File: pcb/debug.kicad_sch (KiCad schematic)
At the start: 23 parts, among them J2 USB_B_Micro, SW1 SW_DIP_x02, U2 FT4222HQ, Y1 12MHz

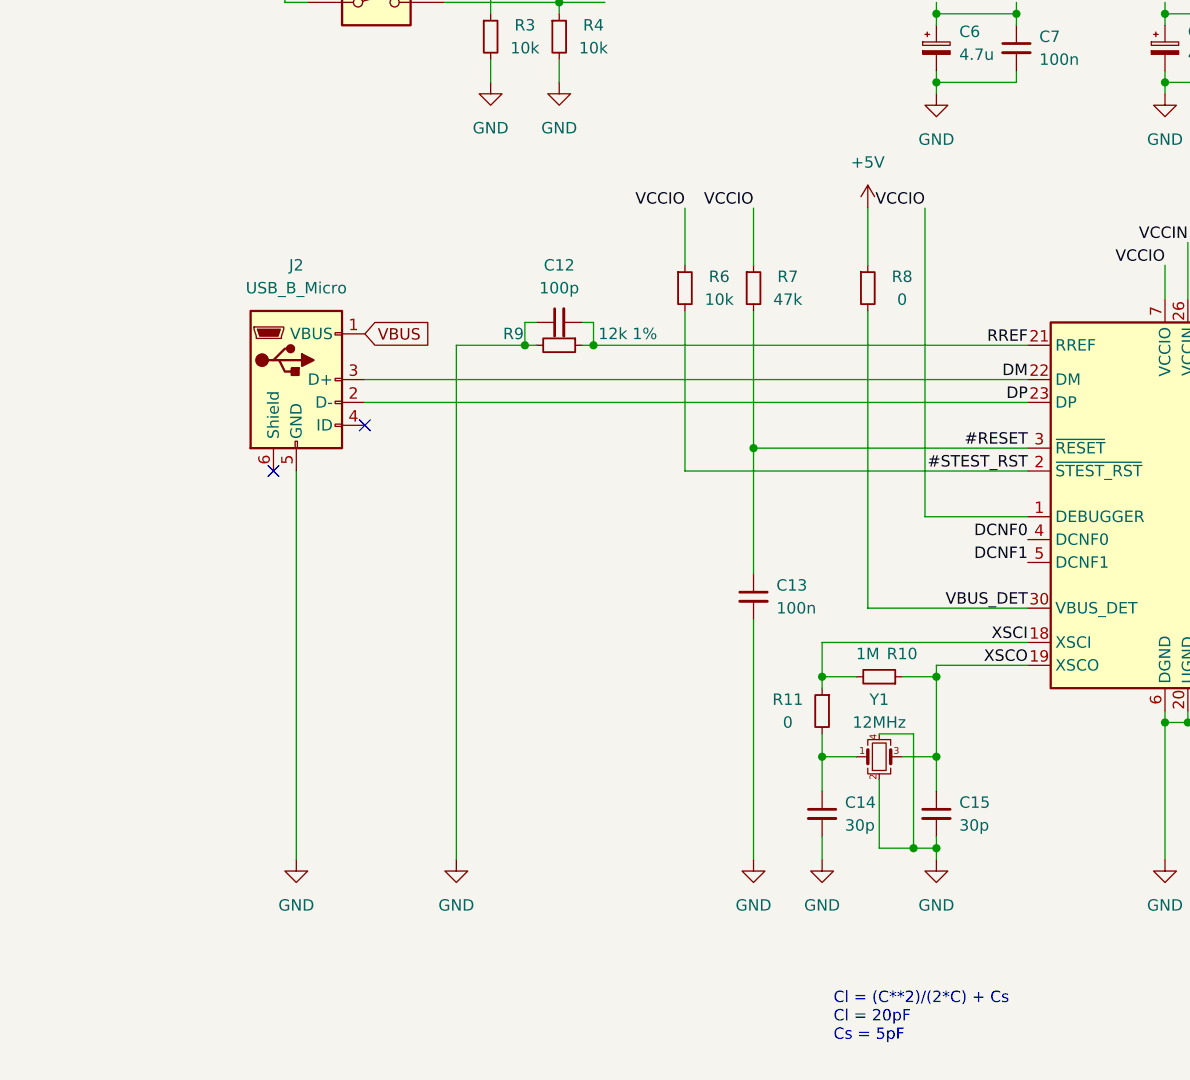
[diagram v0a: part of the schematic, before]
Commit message: add components to the pcb
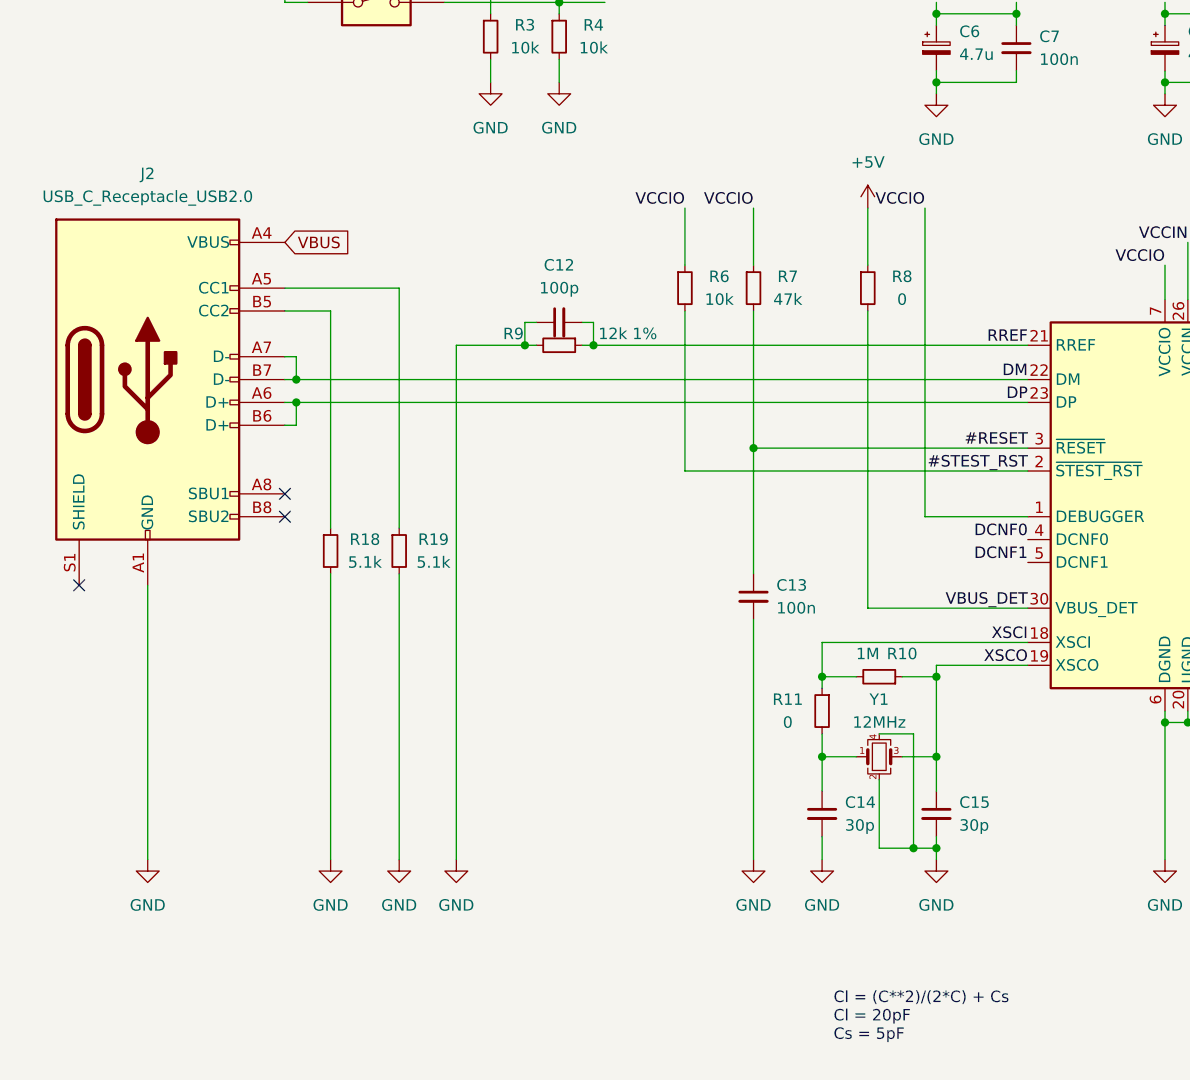
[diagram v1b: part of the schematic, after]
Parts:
- removed J2: USB_B_Micro, 10118194-0001LF:AMPHENOL_10118194-0001LF, symbol Connector:USB_B_Micro
- added J2: USB_C_Receptacle_USB2.0, USB4105-GF-A:GCT_USB4105-GF-A, symbol Connector:USB_C_Receptacle_USB2.0
- added R18, R19: 5.1k, Resistor_SMD:R_0603_1608Metric, symbol Device:R_Small
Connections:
- net DM: now also J2.A7 (D-), J2.B7 (D-)
- net DP: now also J2.A6 (D+), J2.B6 (D+)
- net GND: now also J2.A1 (GND), J2.A12 (GND), J2.B1 (GND), J2.B12 (GND), R18.2, R19.2
- net VBUS: now also J2.A4 (VBUS), J2.A9 (VBUS), J2.B4 (VBUS), J2.B9 (VBUS)
- new net: J2.A5 (CC1), R19.1
- new net: J2.B5 (CC2), R18.1
- no-connect marks 10 -> 11
